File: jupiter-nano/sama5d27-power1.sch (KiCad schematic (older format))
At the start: 1 part, among them U1 ATSAMA5D27C-LD1G-CU

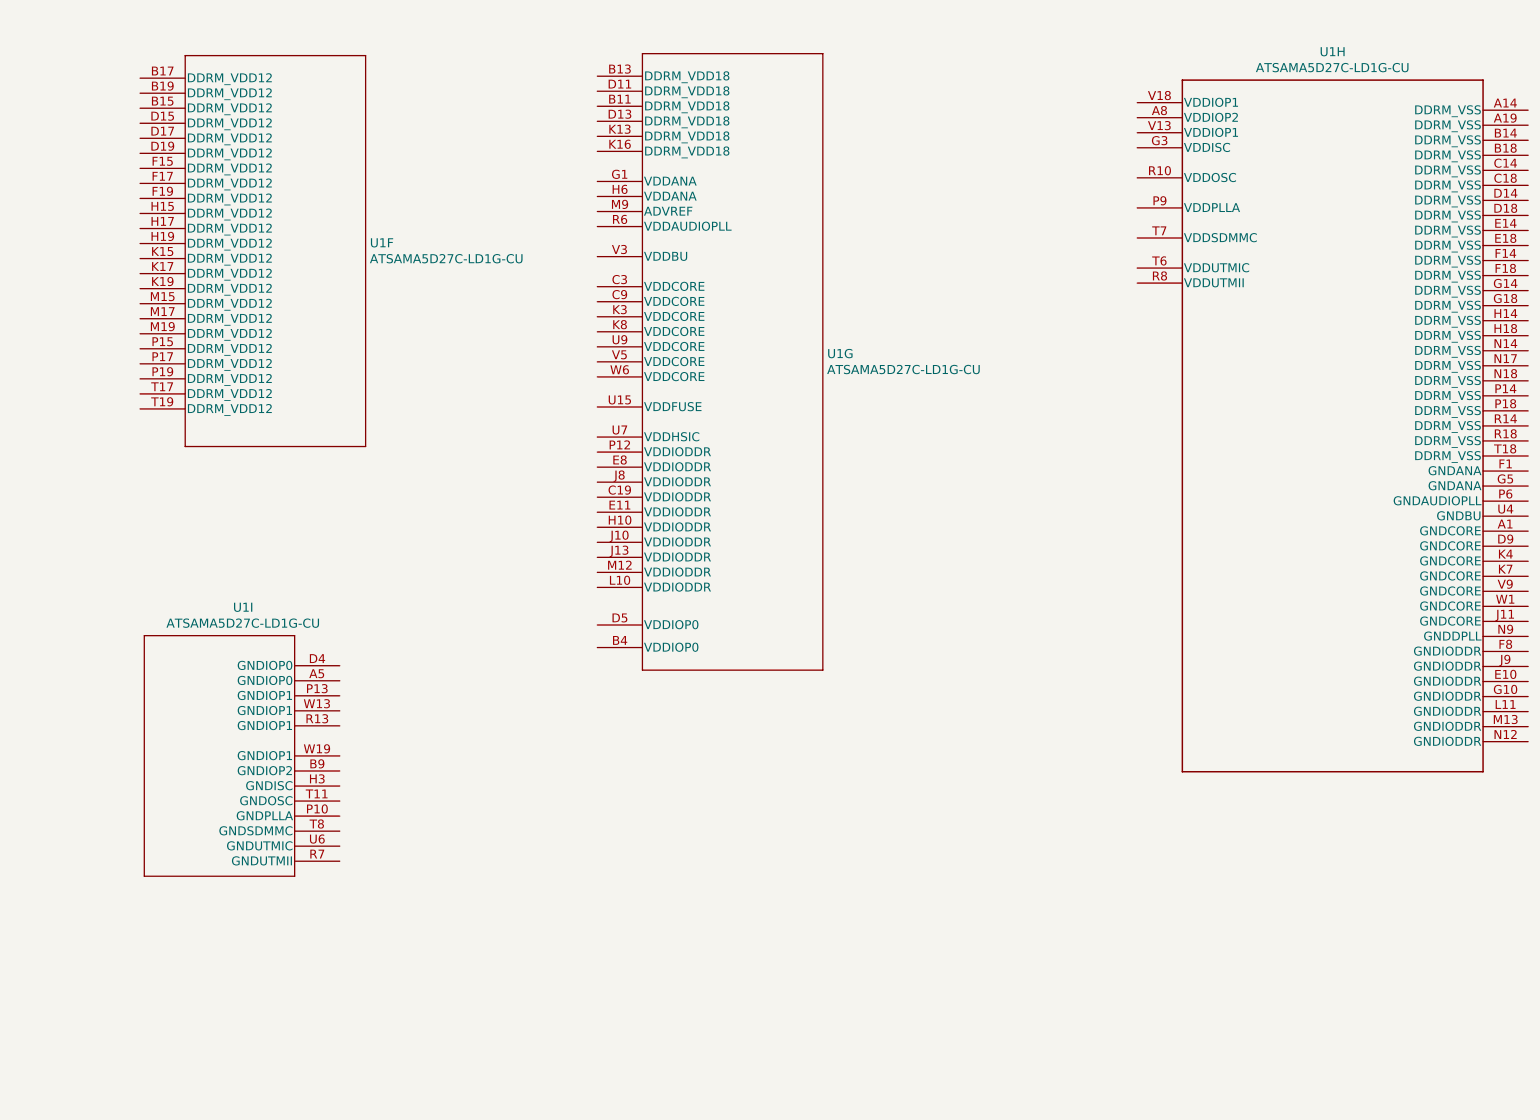
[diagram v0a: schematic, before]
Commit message: WIP – power3 done
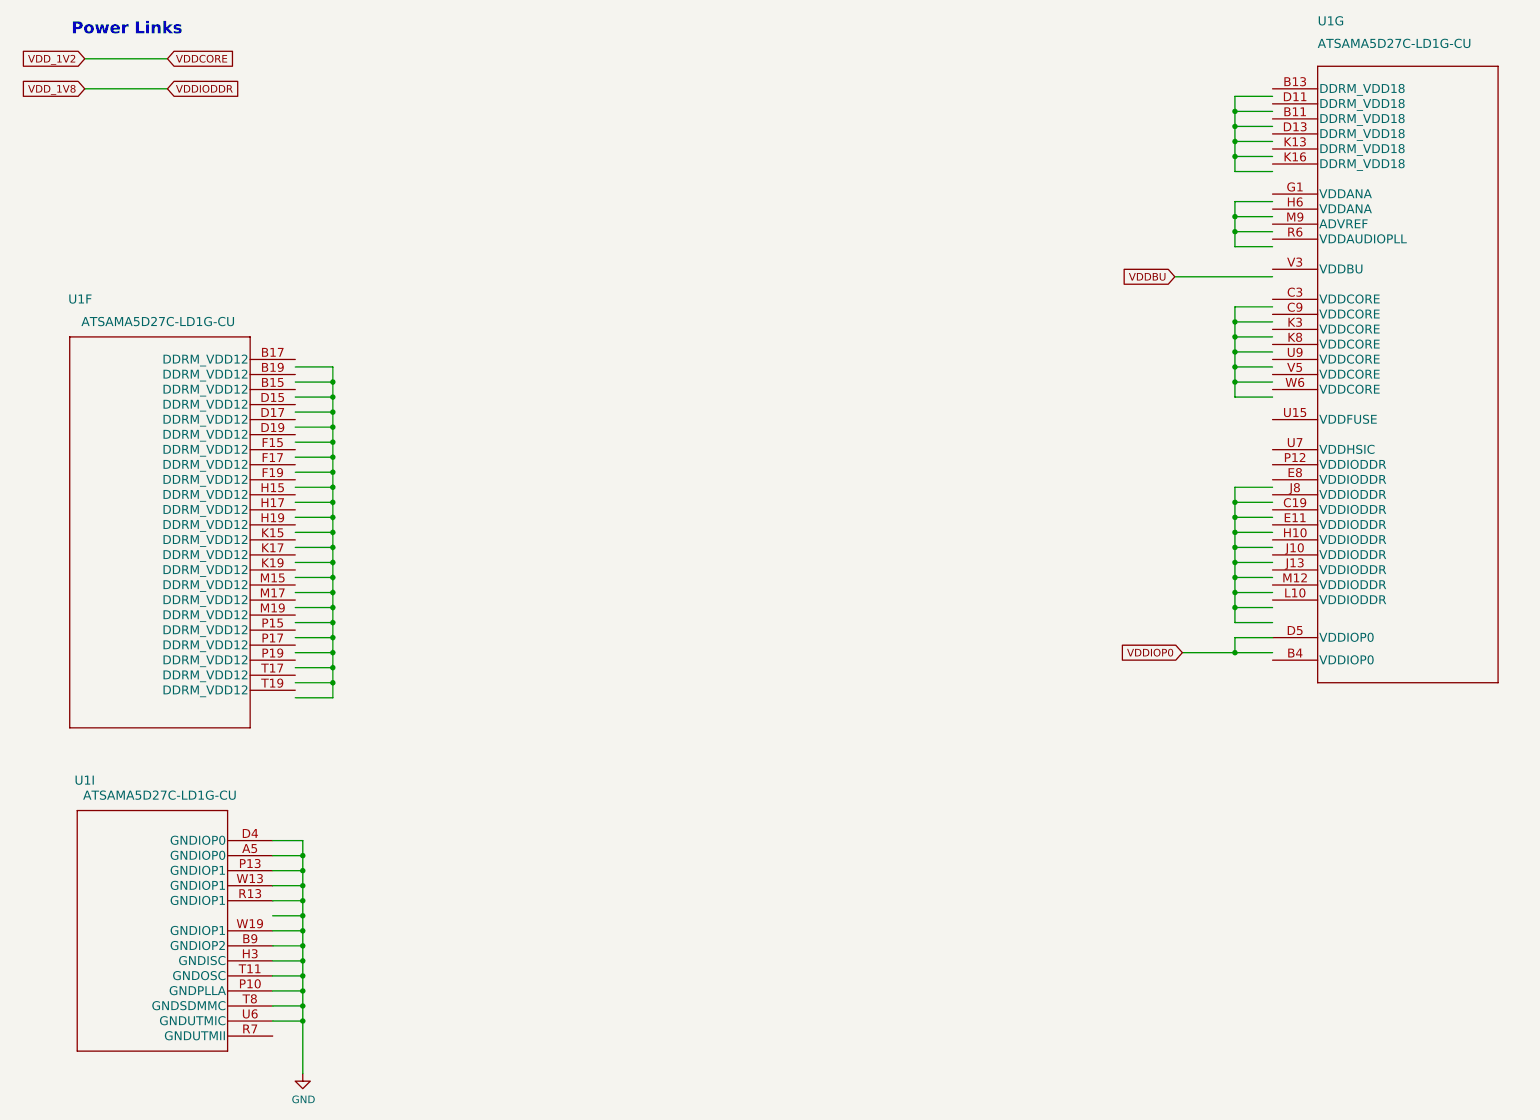
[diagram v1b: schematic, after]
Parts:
- removed unit 8 of U1
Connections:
- net labels added: GND, VDDBU, VDDCORE, VDDIODDR, VDDIOP0, VDD_1V2, VDD_1V8
- wire segments 0 -> 128
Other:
- note added: "Power Links"
- moved on the sheet: U1F, U1G, U1I
